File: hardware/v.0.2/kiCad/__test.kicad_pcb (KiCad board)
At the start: 2 copper layers, 43.5 x 14.3 mm, 34 parts, among them IC1 ATSHA204A, P1 USB_A, P2 1, P3 3, P4 2, SW1 SW_PUSH, SW2 SW_PUSH, SW3 SW_PUSH, SW4 SW_PUSH, SW5 SW_PUSH, U1 STM32F103C8, U2 TLV70033DDC, Y1 Crystal

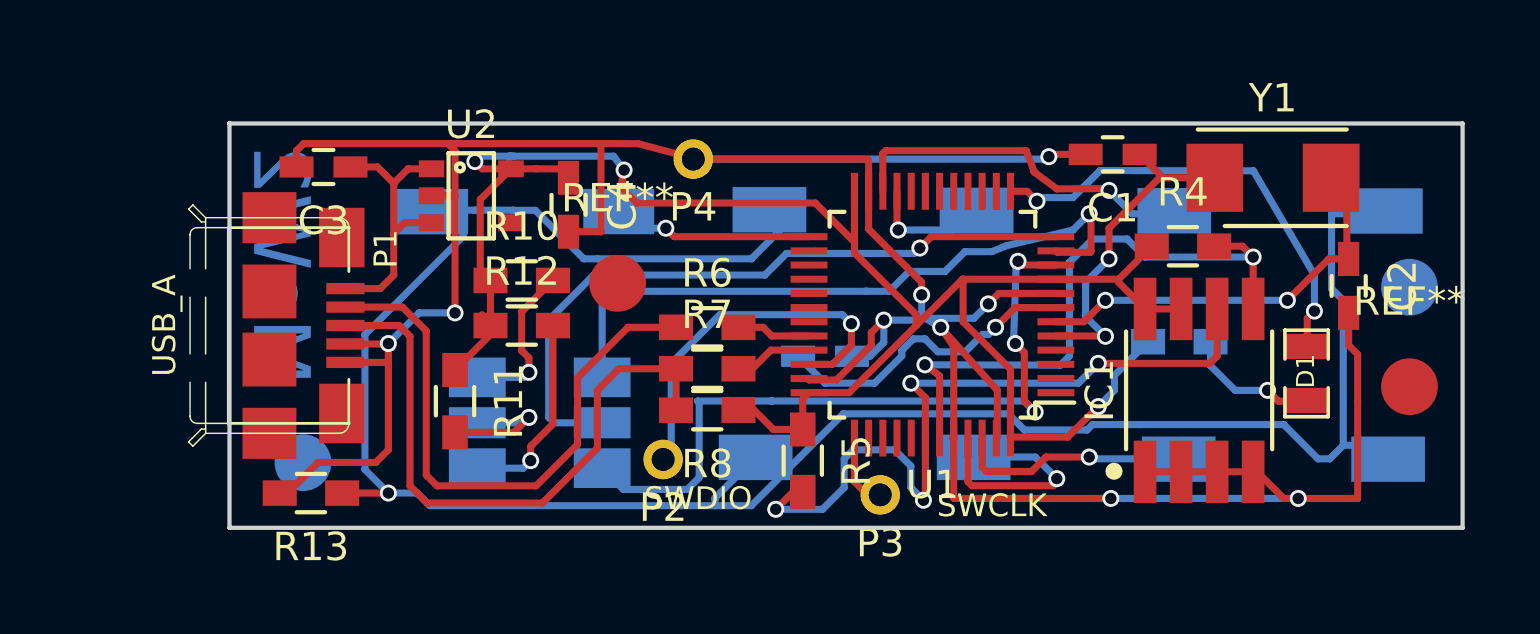
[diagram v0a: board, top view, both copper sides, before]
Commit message: Мелкие правки платы
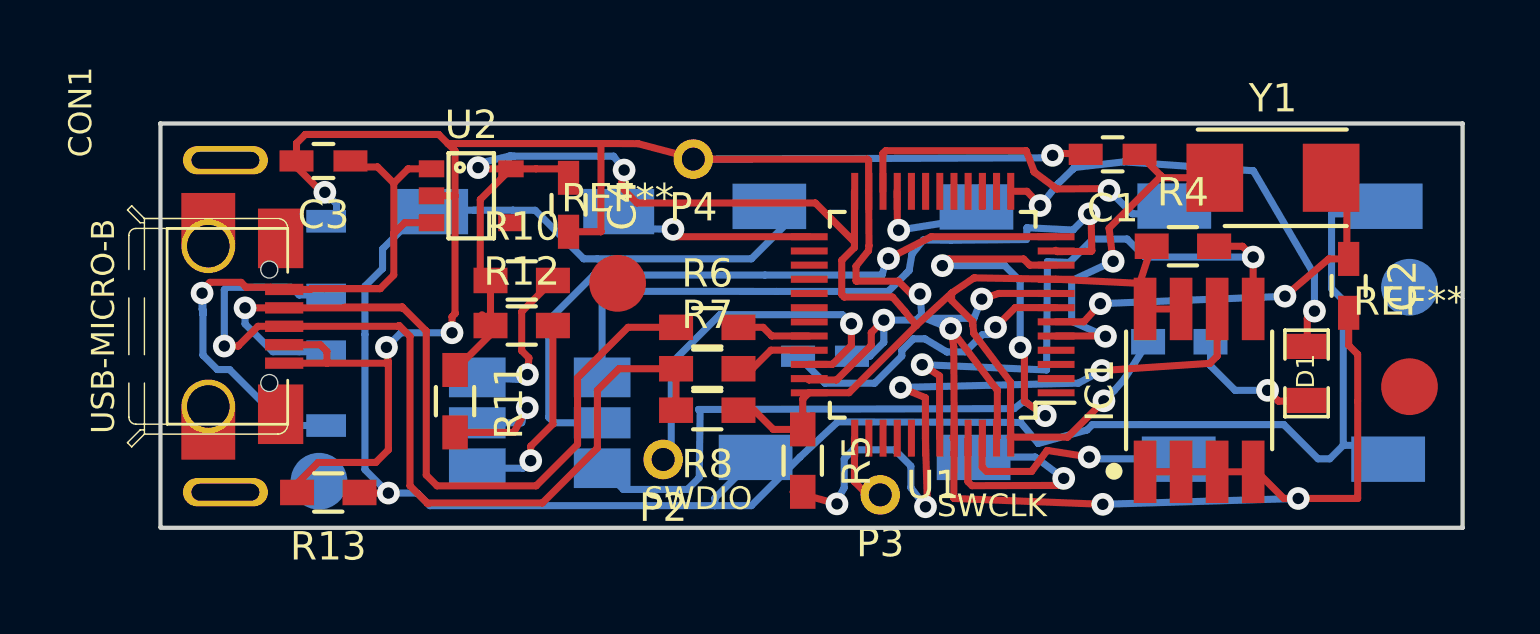
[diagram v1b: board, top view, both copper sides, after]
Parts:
- removed P1: USB_A, user:USB_MICRO_B_SMD
- added CON1: USB-MICRO-B, user:USB_MICRO_B_SMD, F.Cu at (30.4, 36.0)
- added REF**: USB_A, usb-male-A-smd:USB_A, B.Cu at (32.5, 36.0)
- moved REF** 0.86 mm to (34.3, 41.5)
- moved R13 0.61 mm to (34.6, 41.9)
- moved C3 0.21 mm to (34.5, 30.2)
- moved SW4 0.17 mm to (68.1, 31.8)
- moved SW3 0.12 mm to (54.0, 31.8)
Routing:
- net Net-(C3-Pad1): track 9.94 -> 24.8 mm, vias 0 -> 1
- net Net-(P1-Pad3): track 22.0 -> 33.4 mm, vias 0 -> 1
- net Net-(P1-Pad2): track 20.9 -> 30.3 mm, vias 0 -> 1
- net GND: track 118.0 -> 126.0 mm, vias 9 -> 10
- net /LED_B: track 25.8 -> 31.4 mm
- net Net-(C1-Pad1): track 11.8 -> 12.9 mm
- net /LED_R: track 23.7 -> 24.4 mm
- net /I2C_SDA_1: track 21.9 -> 22.4 mm
- net Net-(D2-Pad5): track 4.72 -> 5.24 mm
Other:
- board size 43.5 x 14.3 mm -> 45.9 x 14.2 mm
- net class Default: via_dia 0.6 -> 0.8
- board text removed: "MeW2"
